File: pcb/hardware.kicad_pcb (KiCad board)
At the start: 4 copper layers, 166 parts, among them J1 Micro_SD_Card_Det_Hirose_DM3AT, J2 USB_A, J3 USB_A, U1 AS4C512M16D3L-12BIN, U2 A33, U3 TPS62095RGTR, U4 TPS62095RGTR, U5 TPS62095RGTR, U6 TPS62095RGTR, U7 AP131-25, U8 MPM-15-5, Y1 24Mhz, Y2 32.768khz

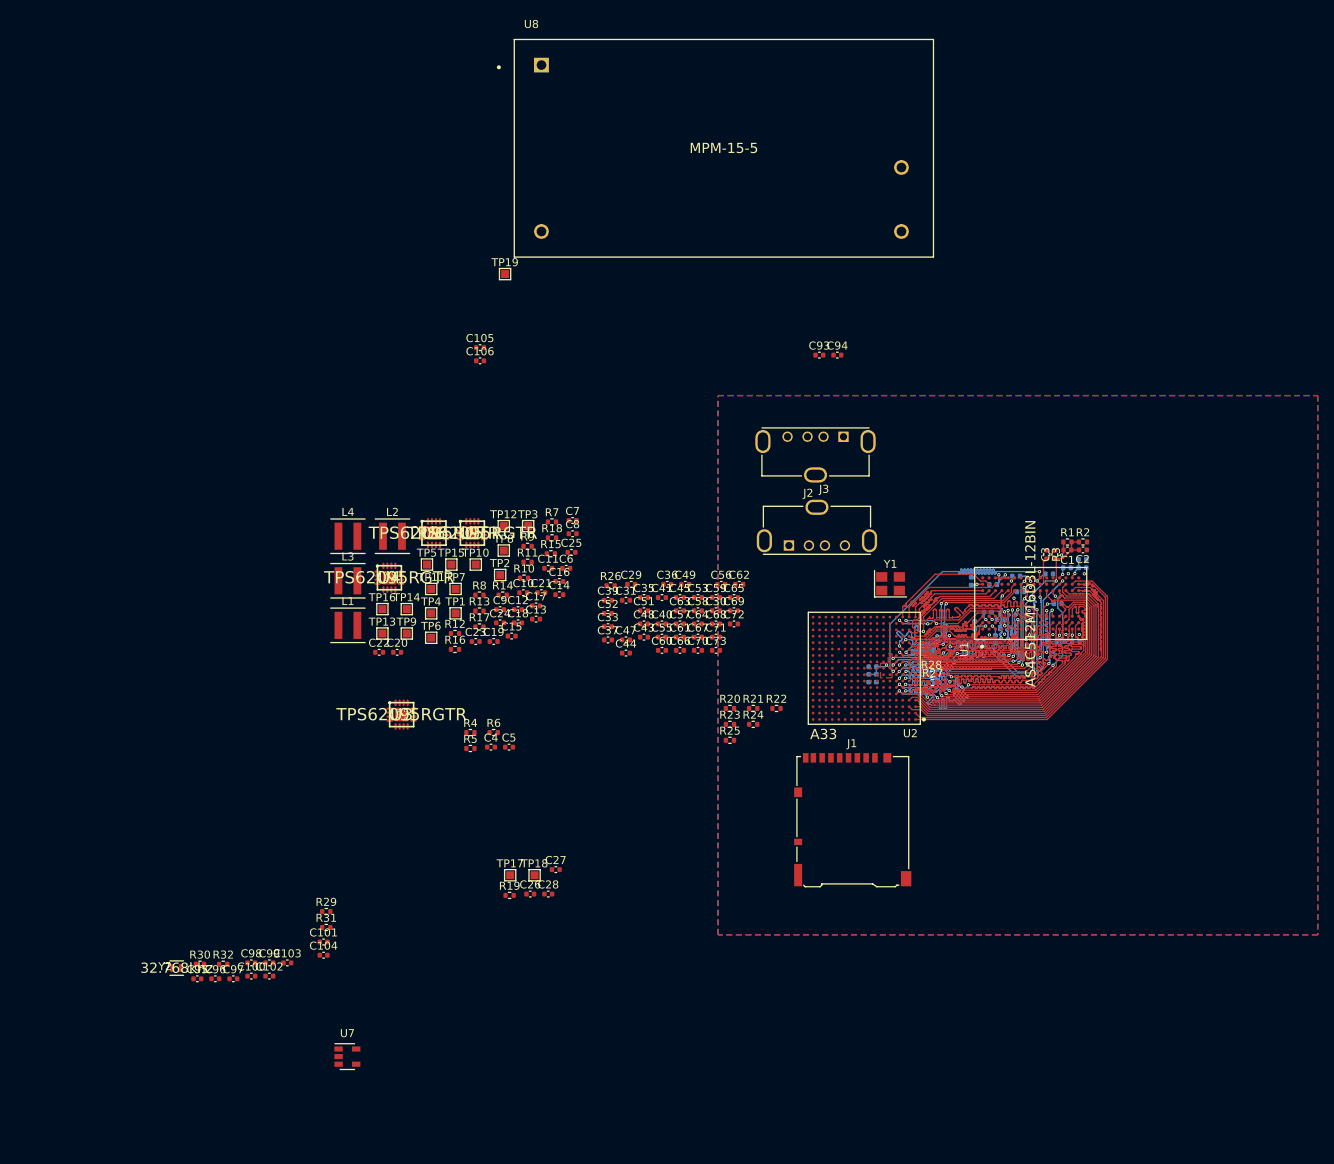
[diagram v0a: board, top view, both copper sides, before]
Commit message: Working on the layout
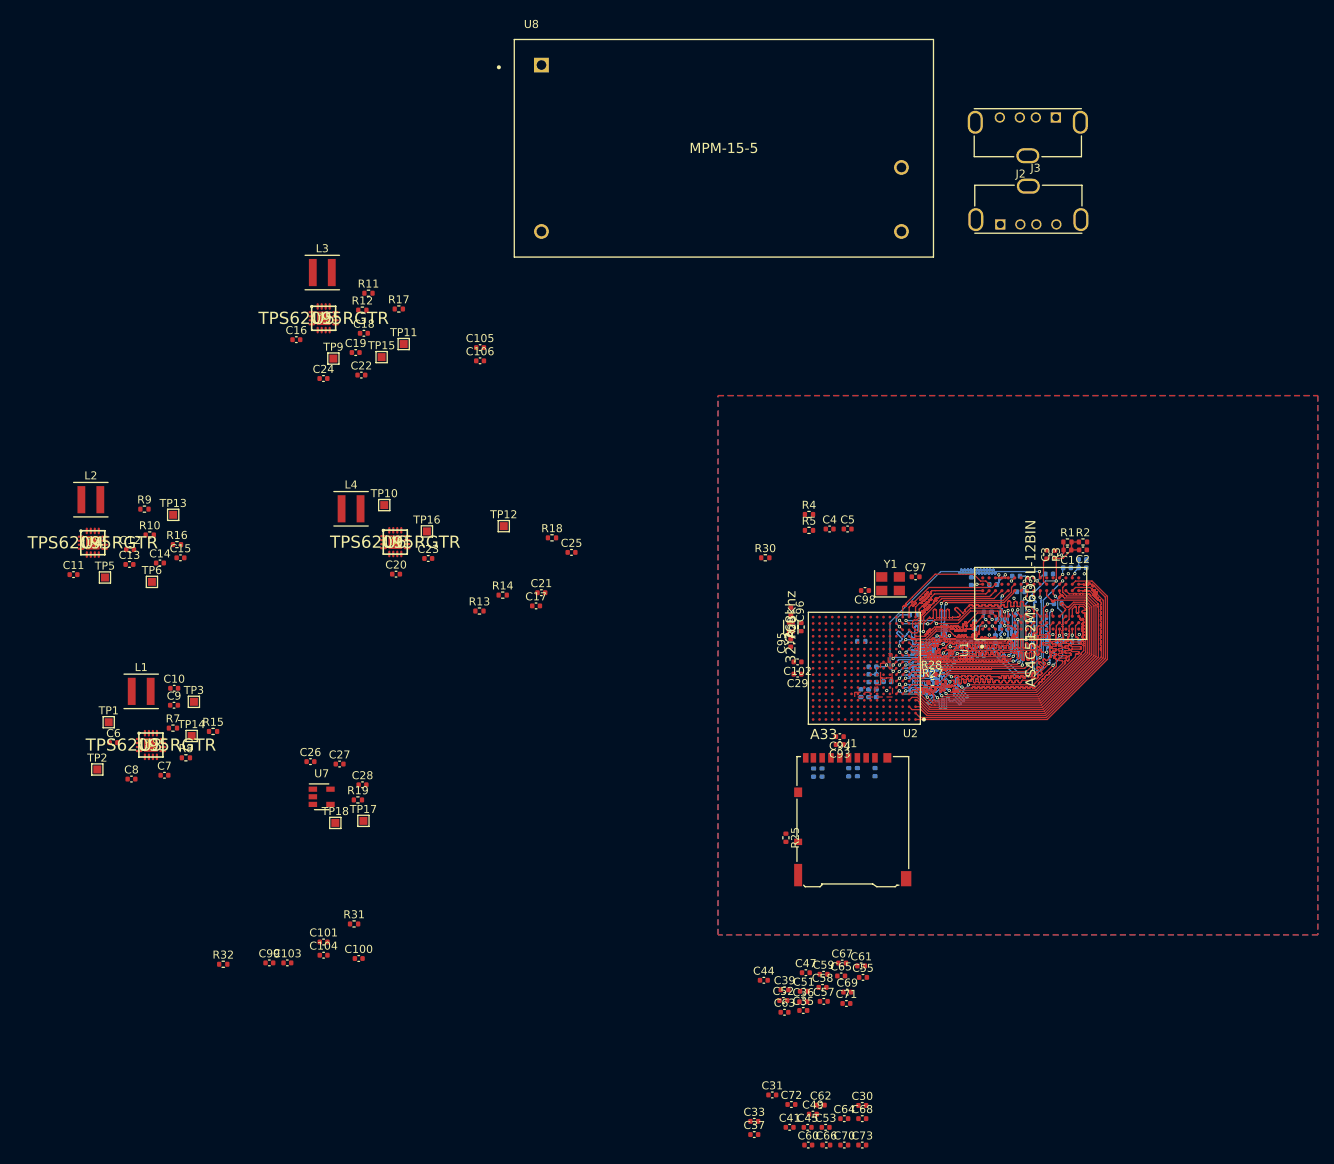
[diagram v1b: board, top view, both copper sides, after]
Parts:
- removed TP19, TP4, TP7, TP8: TestPoint, TestPoint:TestPoint_Pad_1.0x1.0mm
- C40, C43, C48, C56, R20, R21, R22, R23, R24, R26, R6: moved to B.Cu
- moved C97 99.0 mm to (121.2, 97.5)
- moved C98 89.7 mm to (114.8, 99.2), turned to 180 degrees
- moved Y2 87.8 mm to (105.6, 103.8), turned to 90 degrees
- moved R30 87.0 mm to (102.4, 95.2)
- moved C96 85.3 mm to (105.6, 101.9), turned to 270 degrees
- moved C95 85.2 mm to (105.6, 105.8), turned to 90 degrees
- moved C102 76.8 mm to (106.4, 108.2), turned to 180 degrees
- moved R29 69.2 mm to (106.9, 103.8), turned to 90 degrees
- moved C41 68.1 mm to (105.4, 166.3)
- moved C45 68.1 mm to (107.7, 166.3)
- moved C53 68.1 mm to (109.9, 166.3)
- moved C49 68.1 mm to (108.3, 164.7)
- moved C62 65.9 mm to (109.3, 163.6)
- moved C31 64.5 mm to (103.3, 162.3)
- moved C33 64.5 mm to (101.0, 165.6)
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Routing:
- net Net-(R6-Pad1): track 0.00 -> 3.61 mm, vias 0 -> 1
- net +1V1: vias 0 -> 1
- added copper zone on F.Cu, net +1V1
